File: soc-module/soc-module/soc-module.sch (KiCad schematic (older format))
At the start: 13 parts, among them J1 Micro_SD_Card, J2 Conn_01x13, J3 Conn_01x14, SW1 SW_Push, SW2 SW_Push, U1 ATECC608A-SSHDA, U2 ESP32-WROVER-IE-16MB

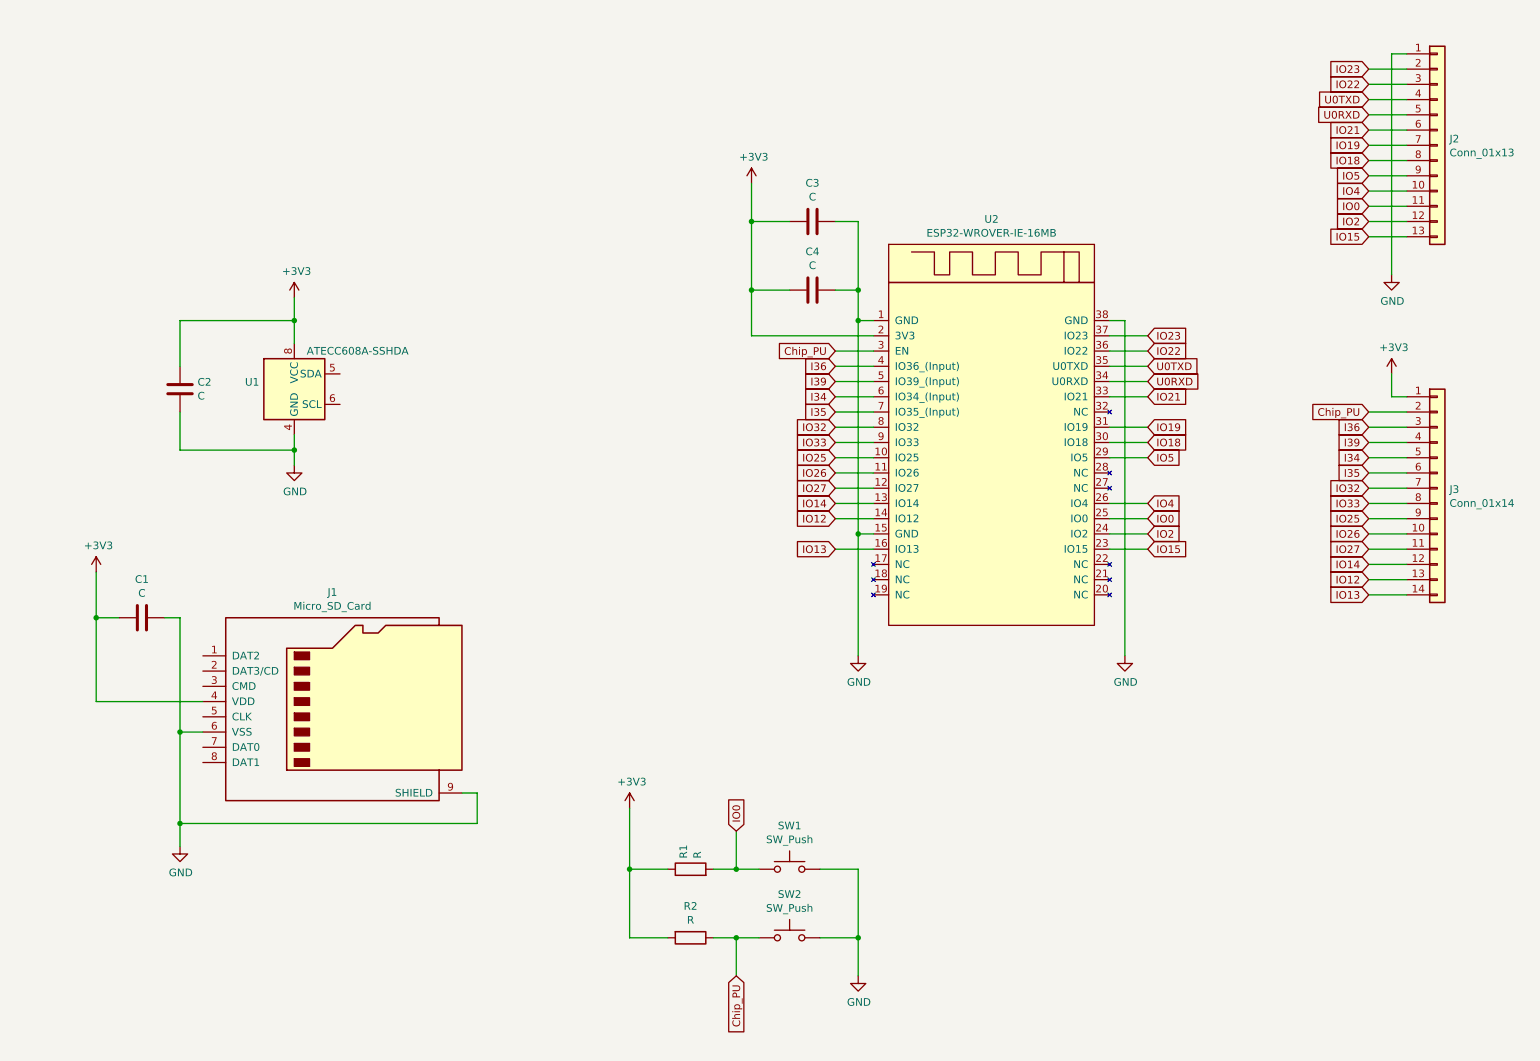
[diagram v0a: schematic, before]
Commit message: SoC Module Work On
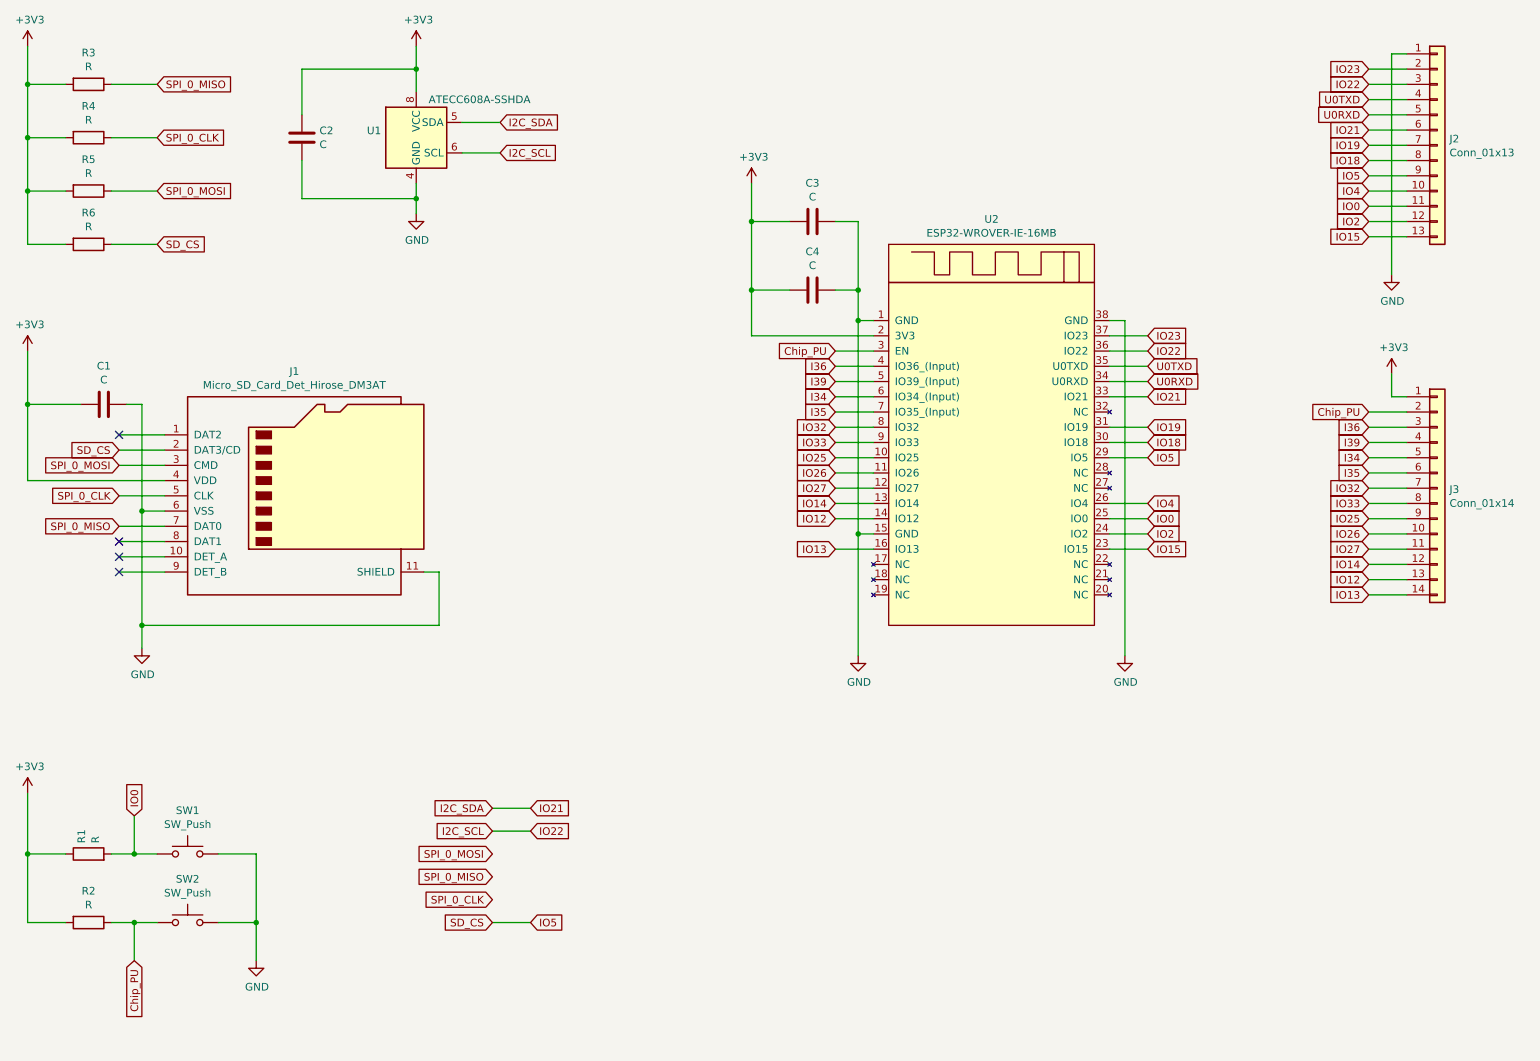
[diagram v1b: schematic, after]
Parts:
- removed J1: Micro_SD_Card, footprints:HRS_DM3AT-SF-PEJM5, symbol Connector:Micro_SD_Card
- added J1: Micro_SD_Card_Det_Hirose_DM3AT, Connector_Card:microSD_HC_Hirose_DM3AT-SF-PEJM5, symbol Connector:Micro_SD_Card_Det_Hirose_DM3AT
- added R3, R4, R5, R6: R, Resistor_SMD:R_1206_3216Metric_Pad1.30x1.75mm_HandSolder, symbol Device:R
- SW1, SW2: footprint (none) -> footprints:SW4SMD_63X161LS
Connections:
- net IO21 is gone; now on net I2C_SDA: J2.6 (Pin_6), U2.33 (IO21)
- net IO22 is gone; now on net I2C_SCL: J2.3 (Pin_3), U2.36 (IO22)
- net +3V3: now also J1.4 (VDD), R3.2, R4.2, R5.2, R6.2
- net GND: now also J1.11 (SHIELD), J1.6 (VSS)
- net IO5: now also J1.2 (DAT3/CD), R6.1
- net I2C_SDA: now reaches U1.5 (SDA)
- net I2C_SCL: now reaches U1.6 (SCL)
- new net SPI_0_CLK: J1.5 (CLK), R4.1
- new net SPI_0_MISO: J1.7 (DAT0), R3.1
- new net SPI_0_MOSI: J1.3 (CMD), R5.1
- no-connect marks 0 -> 4
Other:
- moved on the sheet: C1, C2, R1, R2, SW1, SW2, U1
